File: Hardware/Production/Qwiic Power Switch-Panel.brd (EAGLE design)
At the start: 149.1 x 149.1 mm, 1505 parts, among them J1 Qwiic Right Angle, J10 PTH, J100 PTH, J103 Qwiic Right Angle, J104 PTH, J105 Qwiic Right Angle, J106 PTH, J109 Qwiic Right Angle, J110 PTH, J111 Qwiic Right Angle, J112 PTH, J115 Qwiic Right Angle, J116 PTH, J117 Qwiic Right Angle, J118 PTH, J121 Qwiic Right Angle, J122 PTH, J123 Qwiic Right Angle, J124 PTH, J127 Qwiic Right Angle, J128 PTH, J129 Qwiic Right Angle, J13 Qwiic Right Angle, J130 PTH, J133 Qwiic Right Angle, J134 PTH, J135 Qwiic Right Angle, J136 PTH, J139 Qwiic Right Angle, J14 PTH, J140 PTH, J141 Qwiic Right Angle, J142 PTH, J145 Qwiic Right Angle, J146 PTH, J147 Qwiic Right Angle, J148 PTH, J15 Qwiic Right Angle, J16 PTH, J19 Qwiic Right Angle, J2 PTH, J20 PTH, J21 Qwiic Right Angle, J22 PTH, J25 Qwiic Right Angle, J26 PTH, J27 Qwiic Right Angle, J28 PTH, J3 Qwiic Right Angle, J31 Qwiic Right Angle, J32 PTH, J33 Qwiic Right Angle, J34 PTH, J37 Qwiic Right Angle, J38 PTH, J39 Qwiic Right Angle, J4 PTH, J40 PTH, J43 Qwiic Right Angle, J44 PTH, J45 Qwiic Right Angle, J46 PTH, J49 Qwiic Right Angle, J50 PTH, J51 Qwiic Right Angle, J52 PTH, J55 Qwiic Right Angle, J56 PTH, J57 Qwiic Right Angle, J58 PTH, J61 Qwiic Right Angle, J62 PTH, J63 Qwiic Right Angle, J64 PTH, J67 Qwiic Right Angle, J68 PTH, J69 Qwiic Right Angle, J7 Qwiic Right Angle, J70 PTH, J73 Qwiic Right Angle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

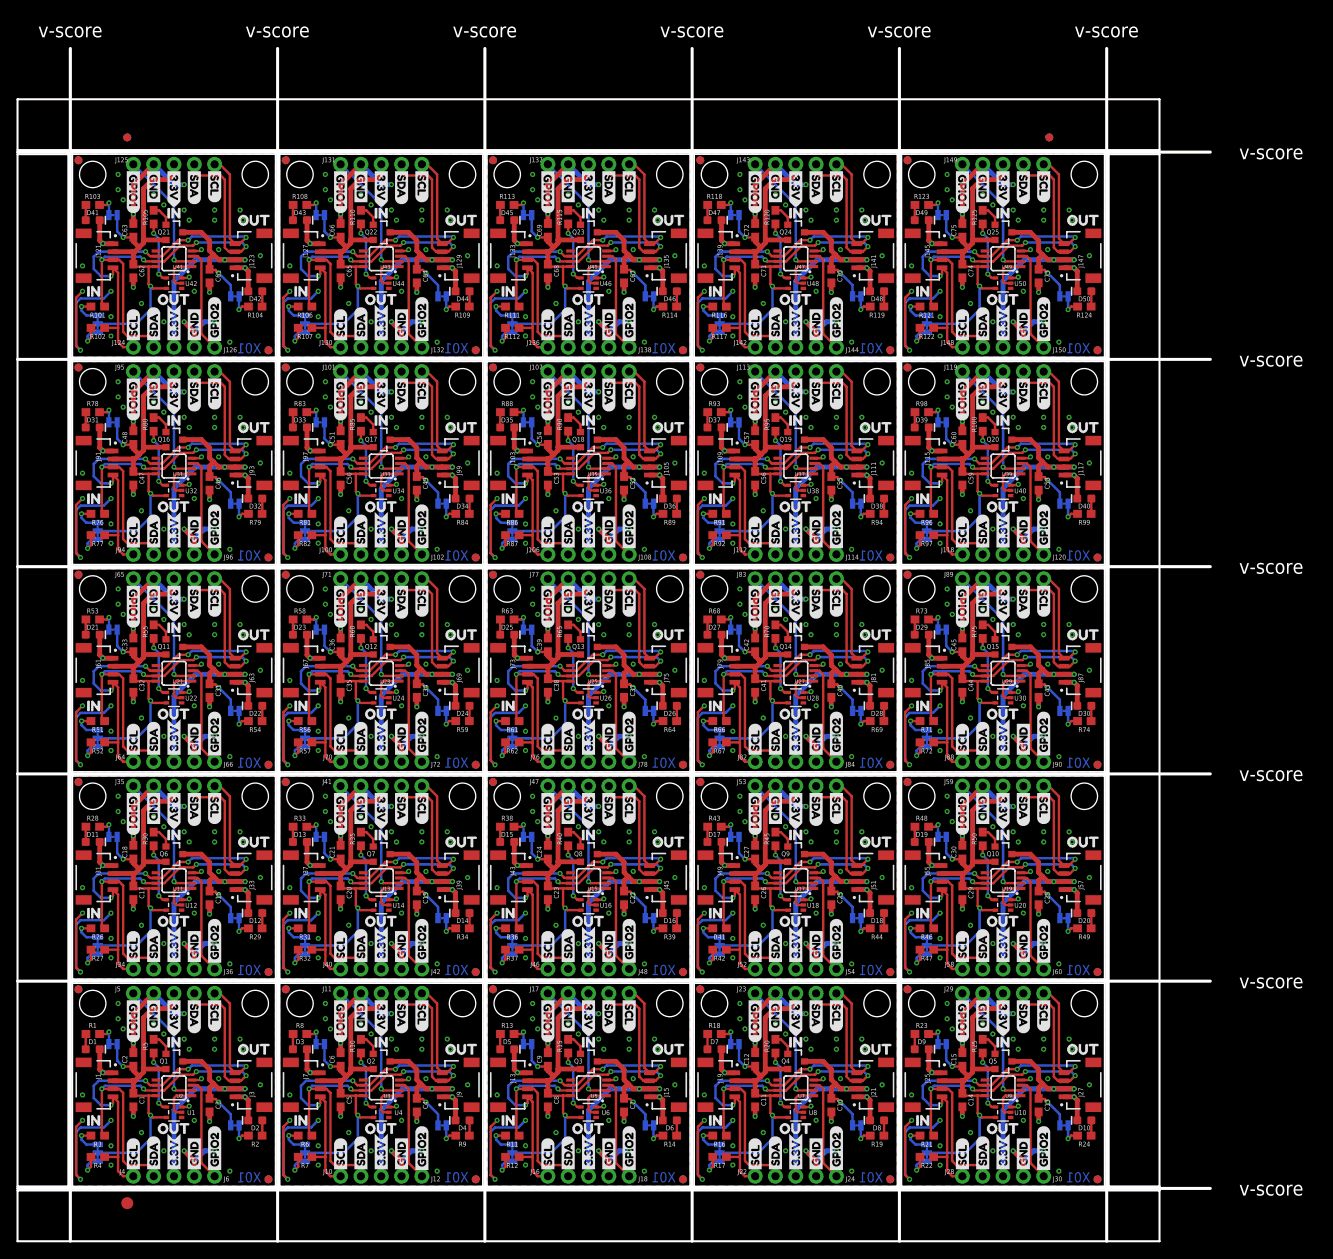
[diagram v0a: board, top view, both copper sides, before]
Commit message: Add x02 production files
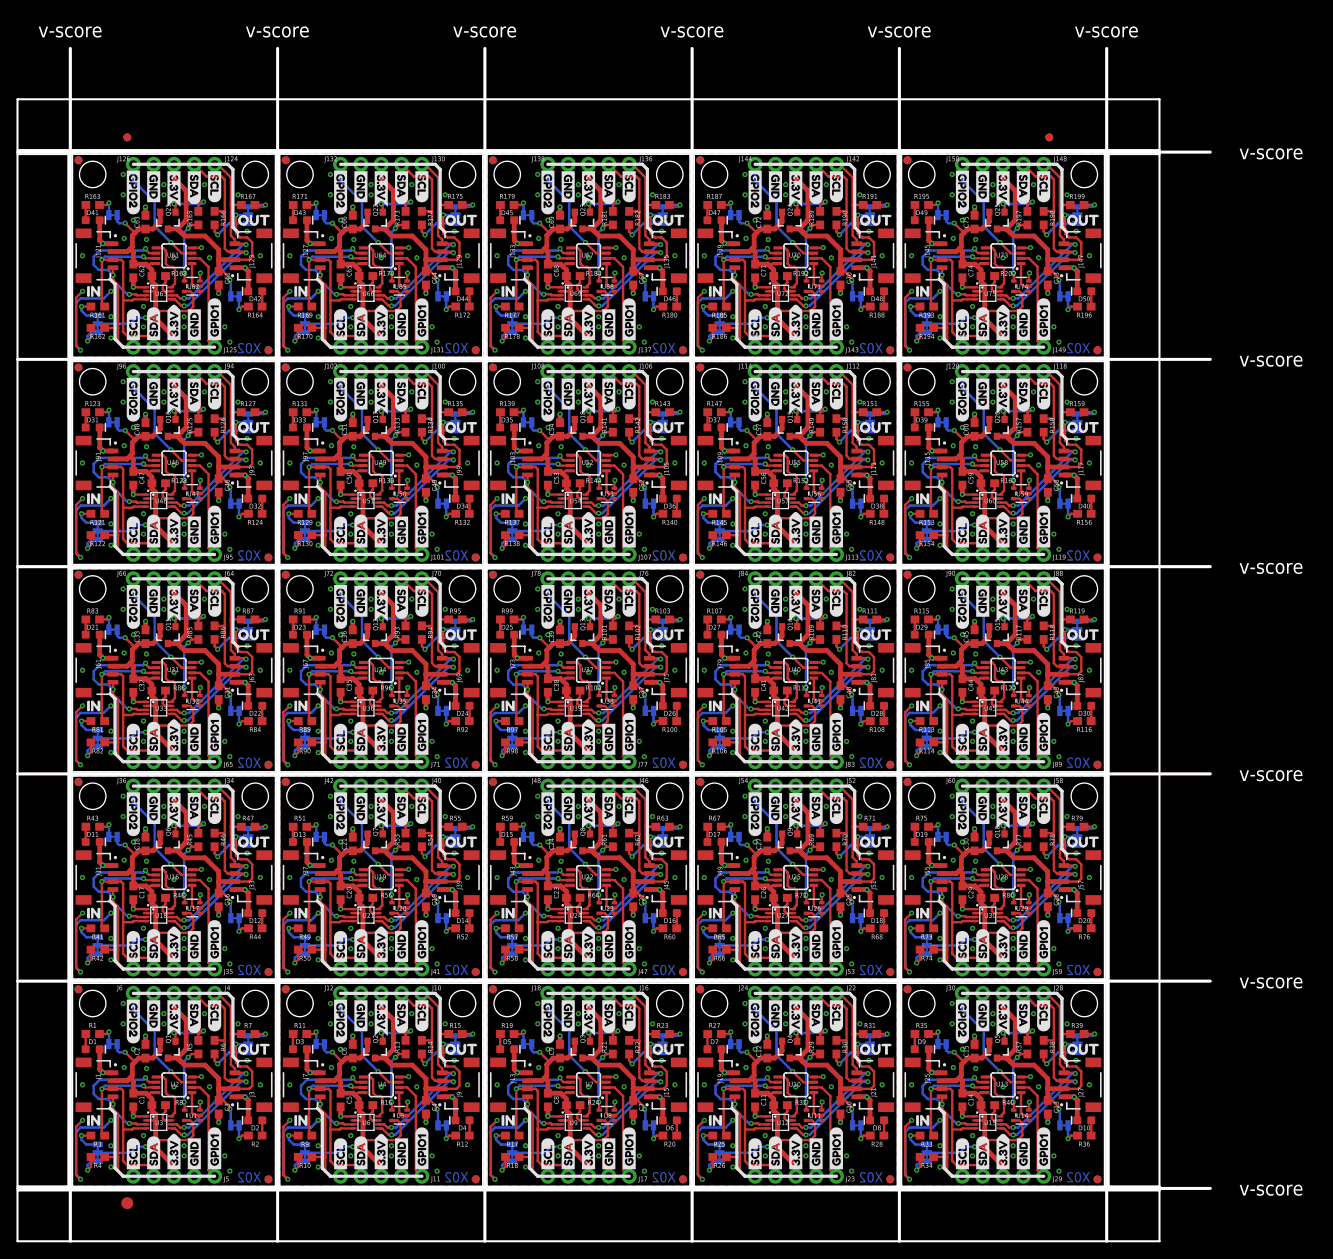
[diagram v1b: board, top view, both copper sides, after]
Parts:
- added I2C_OUT, I2C_OUT1, I2C_OUT10, I2C_OUT11, I2C_OUT12, I2C_OUT13, I2C_OUT14, I2C_OUT15, I2C_OUT16, I2C_OUT17, I2C_OUT18, I2C_OUT19, I2C_OUT2, I2C_OUT20, I2C_OUT21, I2C_OUT22, I2C_OUT23, I2C_OUT24, I2C_OUT3, I2C_OUT4, I2C_OUT5, I2C_OUT6, I2C_OUT7, I2C_OUT8, I2C_OUT9: JUMPER-SMT_3_2-NC_TRACE_SILK, SparkFun-Jumpers:SMT-JUMPER_3_2-NC_TRACE_SILK
- added R126, R127, R129, R130, R134, R135, R137, R138, R142, R143, R145, R146, R150, R151, R153, R154, R158, R159, R161, R162, R166, R167, R169, R170, R174, R175, R177, R178, R182, R183, R185, R186, R190, R191, R193, R194, R198, R199: 2.2k, SparkFun-Resistors:0603
- added R128, R136, R144, R152, R160, R168, R176, R184, R192, R200: 200k, SparkFun-Resistors:0603
- added R131, R133, R139, R141, R147, R149, R155, R157, R163, R165, R171, R173, R179, R181, R187, R189, R195, R197: 1k, SparkFun-Resistors:0603
- added R132, R140, R148, R156, R164, R172, R180, R188, R196: 470, SparkFun-Resistors:0603
- added U$776, U$800: (no value), Labels:I_SUPER2_C-()-03
- added U$777, U$780: (no value), Labels-0_04:GND1
- added U$778, U$782: (no value), Labels-0_04:SCL9
- added U$779, U$781: (no value), Labels-0_04:SDA8
- added U$783: (no value), Qwiic:QWIIC0
- added U$784, U$797: (no value), 3.3V_Flagtail:3#3V0
- added U$785, U$796: (no value), 3.3V_Pointer:3#3V0
- added U$786, U$794: (no value), GPIO1:GPIO10
- added U$787, U$795: (no value), GPIO2:GPIO20
- added U$788: (no value), IN:IN0
- added U$789: (no value), LED_IN:LED_IN0
- added U$790: (no value), LED_OUT:LED_OUT0
- added U$791: (no value), OUT:OUT0
- added U$792: (no value), Power:POWER0
- added U$793: (no value), Switch:SWITCH0
- added U$798: (no value), IN__3:IN0
- added U$799: (no value), OUT__3:OUT0
- added U51, U54, U57, U60, U63, U66, U69, U72, U75: (no value), SparkFun-IC-Comms:VSSOP_8PIN
- added U52, U55, U58, U61, U64, U67, U70, U73: PCA9536, New_Parts:MSOP8
- added U53, U56, U59, U62, U65, U68, U71, U74: 74HC1G04, SparkFun-IC-Logic:SOT353
- R10, R103, R105, R110, R113, R114, R118, R119, R14, R15, R18, R23, R25, R30, R33, R34, R38, R39, R49, R50, R54, R55, R58, R63, R65, R70, R73, R74, R78, R79, R89, R9, R90, R94, R95, R98: value 1k -> 2.2k
- R100, R108, R124, R2, R20, R28, R44, R60, R68, R84: value 1k -> 470
- R101, R107, R11, R117, R21, R27, R37, R51, R61, R67, R77, R91: value 2.2k -> 1k
- R104, R120, R24, R40, R48, R64, R8, R80, R88: value 1k -> 200k
- R112, R16, R32, R56, R72, R96: value 2.2k -> 200k
- R116, R12, R36, R52, R76, R92: value 2.2k -> 470
- U$1, U$94: value SPARKX-LOGO4 -> (none); device SparkX:SPARKX-MEDIUM -> IN__3:IN0
- U$100, U$107, U$134, U$196, U$262, U$324, U$38, U$45, U$685, U$747: device Labels-0_04:SCL9 -> Labels-0_04:SDA8
- U$101, U$194: device Labels:I_SUPER2_C-()-03 -> Labels-0_04:GND1
- U$102, U$164, U$198, U$260, U$36, U$43, U$653, U$715, U$749: device Labels-0_04:GND1 -> Labels-0_04:SDA8
- U$104, U$128, U$168, U$192, U$352, U$416: device Labels-0_04:SDA8 -> Labels:I_SUPER2_C-()-03
- U$106, U$135, U$199, U$259, U$323, U$35, U$42, U$686, U$750, U$99: device Labels-0_04:SDA8 -> Labels-0_04:SCL9
- U$108, U$201, U$325, U$418: device Qwiic:QWIIC0 -> Labels-0_04:GND1
- U$109, U$171, U$326, U$388, U$525, U$587, U$742: device 3.3V_Flagtail:3#3V0 -> Labels-0_04:SDA8
- U$110, U$234, U$327, U$451, U$462, U$586, U$679: device 3.3V_Pointer:3#3V0 -> Labels-0_04:SCL9
- U$111, U$367: device GPIO1:GPIO10 -> Qwiic:QWIIC0
- U$112, U$368, U$701: device GPIO2:GPIO20 -> 3.3V_Flagtail:3#3V0
- U$113, U$433, U$764, U$92: device IN:IN0 -> 3.3V_Pointer:3#3V0
- U$114: device LED_IN:LED_IN0 -> GPIO1:GPIO10
- U$115: device LED_OUT:LED_OUT0 -> GPIO2:GPIO20
- U$116, U$372: device OUT:OUT0 -> IN:IN0
- U$117: device Power:POWER0 -> LED_IN:LED_IN0
- U$118: device Switch:SWITCH0 -> LED_OUT:LED_OUT0
- U$119: device GPIO1:GPIO10 -> OUT:OUT0
- U$120: device GPIO2:GPIO20 -> Power:POWER0
- U$121, U$761: device 3.3V_Pointer:3#3V0 -> Switch:SWITCH0
- U$122, U$370, U$698: device 3.3V_Flagtail:3#3V0 -> GPIO1:GPIO10
- U$123, U$371, U$51: device IN:IN0 -> GPIO2:GPIO20
- U$124, U$209, U$465: device OUT:OUT0 -> 3.3V_Pointer:3#3V0
- U$125, U$528: value SPARKX-LOGO4 -> (none); device SparkX:SPARKX-MEDIUM -> 3.3V_Flagtail:3#3V0
- U$126, U$222, U$350, U$446: device Labels-0_04:GND1 -> IN__3:IN0
- U$127, U$255, U$351, U$479: device Labels-0_04:SCL9 -> OUT__3:OUT0
- U$129, U$257, U$353: value (none) -> SPARKX-LOGO4; device Labels-0_04:GND1 -> SparkX:SPARKX-MEDIUM
- U$130, U$137, U$197, U$261, U$290, U$354, U$37, U$44, U$66, U$73, U$748: device Labels-0_04:SDA8 -> Labels-0_04:GND1
- U$132, U$70: device Labels:I_SUPER2_C-()-03 -> Labels-0_04:SDA8
- U$136, U$160, U$18, U$288, U$384, U$40, U$64: device Labels-0_04:GND1 -> Labels:I_SUPER2_C-()-03
- U$139, U$294, U$356, U$77: device Qwiic:QWIIC0 -> Labels-0_04:SDA8
- U$14, U$671: device IN:IN0 -> OUT__3:OUT0
- U$140, U$233, U$357, U$450, U$556, U$649, U$773: device 3.3V_Flagtail:3#3V0 -> Labels-0_04:GND1
- U$141, U$203, U$358, U$420, U$493, U$555, U$710, U$772: device 3.3V_Pointer:3#3V0 -> Labels-0_04:SDA8
- U$142, U$266, U$359, U$398, U$483, U$522, U$615, U$739: device GPIO1:GPIO10 -> Labels-0_04:SCL9
- U$143, U$399: device GPIO2:GPIO20 -> Qwiic:QWIIC0
- U$144, U$464, U$61, U$733: device IN:IN0 -> 3.3V_Flagtail:3#3V0
- U$145: device LED_IN:LED_IN0 -> 3.3V_Pointer:3#3V0
- U$146: device LED_OUT:LED_OUT0 -> GPIO1:GPIO10
- U$147, U$155, U$403: device OUT:OUT0 -> GPIO2:GPIO20
- U$148: device Power:POWER0 -> IN:IN0
- U$149: device Switch:SWITCH0 -> LED_IN:LED_IN0
- U$150: device GPIO1:GPIO10 -> LED_OUT:LED_OUT0
- U$151: device GPIO2:GPIO20 -> OUT:OUT0
- U$152: device 3.3V_Pointer:3#3V0 -> Power:POWER0
- U$153, U$729: device 3.3V_Flagtail:3#3V0 -> Switch:SWITCH0
- U$154, U$402, U$82: device IN:IN0 -> GPIO1:GPIO10
- U$156, U$497: value SPARKX-LOGO4 -> (none); device SparkX:SPARKX-MEDIUM -> 3.3V_Pointer:3#3V0
- U$157, U$253, U$381, U$477, U$560, U$656: device Labels-0_04:GND1 -> 3.3V_Flagtail:3#3V0
- U$158, U$286, U$382, U$510: device Labels-0_04:SCL9 -> IN__3:IN0
- U$159, U$223, U$383, U$447: device Labels-0_04:SDA8 -> OUT__3:OUT0
- U$161, U$321, U$385, U$97: value (none) -> SPARKX-LOGO4; device Labels-0_04:SDA8 -> SparkX:SPARKX-MEDIUM
- U$162, U$165, U$169, U$258, U$293, U$33, U$386, U$41, U$69, U$716, U$76: device Labels-0_04:SCL9 -> Labels-0_04:GND1
- U$163, U$39: device Labels:I_SUPER2_C-()-03 -> Labels-0_04:SCL9
- U$167, U$195, U$291, U$622, U$67, U$71, U$718, U$74, U$746: device Labels-0_04:GND1 -> Labels-0_04:SCL9
- U$170, U$263, U$387, U$46: device Qwiic:QWIIC0 -> Labels-0_04:SCL9
- U$172, U$265, U$389, U$482, U$524, U$617, U$741: device 3.3V_Pointer:3#3V0 -> Labels-0_04:GND1
- U$173, U$235, U$390, U$429, U$452, U$491, U$646, U$708: device GPIO1:GPIO10 -> Labels-0_04:SDA8
- U$174, U$298, U$391, U$430, U$515, U$554, U$647, U$771: device GPIO2:GPIO20 -> Labels-0_04:SCL9
- U$175, U$495: device IN:IN0 -> Qwiic:QWIIC0
- U$176, U$765: device LED_IN:LED_IN0 -> 3.3V_Flagtail:3#3V0
- U$177: device LED_OUT:LED_OUT0 -> 3.3V_Pointer:3#3V0
- U$178, U$186, U$434: device OUT:OUT0 -> GPIO1:GPIO10
- U$179: device Power:POWER0 -> GPIO2:GPIO20
- U$180: device Switch:SWITCH0 -> IN:IN0
- U$181: device GPIO1:GPIO10 -> LED_IN:LED_IN0
- U$182: device GPIO2:GPIO20 -> LED_OUT:LED_OUT0
- U$183: device 3.3V_Pointer:3#3V0 -> OUT:OUT0
- U$184, U$760: device 3.3V_Flagtail:3#3V0 -> Power:POWER0
- U$185: device IN:IN0 -> Switch:SWITCH0
- U$187, U$435: value SPARKX-LOGO4 -> (none); device SparkX:SPARKX-MEDIUM -> GPIO2:GPIO20
- U$188, U$284, U$412, U$508, U$529, U$625, U$753: device Labels-0_04:GND1 -> 3.3V_Pointer:3#3V0
- U$189, U$317, U$413, U$541, U$592, U$720: device Labels-0_04:SCL9 -> 3.3V_Flagtail:3#3V0
- U$190, U$254, U$414, U$478: device Labels-0_04:SDA8 -> IN__3:IN0
- U$191, U$319, U$415, U$95: device Labels-0_04:GND1 -> OUT__3:OUT0
- U$193, U$289, U$417, U$65: value (none) -> SPARKX-LOGO4; device Labels-0_04:SCL9 -> SparkX:SPARKX-MEDIUM
- U$200, U$224, U$320, U$448, U$72, U$96: device Labels-0_04:SCL9 -> Labels:I_SUPER2_C-()-03
- U$202, U$295, U$419, U$494, U$618, U$711, U$78: device 3.3V_Flagtail:3#3V0 -> Labels-0_04:SCL9
- U$204, U$297, U$421, U$460, U$514, U$553, U$677, U$770: device GPIO1:GPIO10 -> Labels-0_04:GND1
- U$205, U$267, U$422, U$461, U$484, U$523, U$678, U$740: device GPIO2:GPIO20 -> Labels-0_04:SDA8
- U$206, U$330, U$423, U$526, U$547, U$650, U$743: device IN:IN0 -> Labels-0_04:SCL9
- U$207: device LED_IN:LED_IN0 -> Qwiic:QWIIC0
- U$208: device LED_OUT:LED_OUT0 -> 3.3V_Flagtail:3#3V0
- U$21, U$705: value (none) -> SPARKX-LOGO4; device OUT:OUT0 -> SparkX:SPARKX-MEDIUM
- U$210: device Power:POWER0 -> GPIO1:GPIO10
- U$211: device Switch:SWITCH0 -> GPIO2:GPIO20
- U$212: device GPIO1:GPIO10 -> IN:IN0
- U$213: device GPIO2:GPIO20 -> LED_IN:LED_IN0
- U$214: device 3.3V_Pointer:3#3V0 -> LED_OUT:LED_OUT0
- U$215: device 3.3V_Flagtail:3#3V0 -> OUT:OUT0
- U$216: device IN:IN0 -> Power:POWER0
- U$217: device OUT:OUT0 -> Switch:SWITCH0
- U$218, U$466: value SPARKX-LOGO4 -> (none); device SparkX:SPARKX-MEDIUM -> GPIO1:GPIO10
- U$219, U$315, U$443, U$467, U$539, U$563, U$691: device Labels-0_04:GND1 -> GPIO2:GPIO20
- U$220, U$348, U$444, U$561, U$572, U$689: device Labels-0_04:SCL9 -> 3.3V_Pointer:3#3V0
- U$221, U$285, U$445, U$509, U$624, U$688: device Labels-0_04:SDA8 -> 3.3V_Flagtail:3#3V0
- U$225: value (none) -> SPARKX-LOGO4; device Labels:I_SUPER2_C-()-03 -> SparkX:SPARKX-MEDIUM
- U$232, U$480: device Qwiic:QWIIC0 -> Labels:I_SUPER2_C-()-03
- U$236, U$329, U$453, U$492, U$546, U$585, U$709: device GPIO2:GPIO20 -> Labels-0_04:GND1
- U$237, U$299, U$454, U$516, U$557, U$619, U$774: device IN:IN0 -> Labels-0_04:SDA8
- U$238, U$362, U$455, U$579: device LED_IN:LED_IN0 -> Labels-0_04:SCL9
- U$239: device LED_OUT:LED_OUT0 -> Qwiic:QWIIC0
- U$240, U$496, U$93: device OUT:OUT0 -> 3.3V_Flagtail:3#3V0
- U$241: device Power:POWER0 -> 3.3V_Pointer:3#3V0
- U$242: device Switch:SWITCH0 -> GPIO1:GPIO10
- U$243, U$731: device GPIO1:GPIO10 -> GPIO2:GPIO20
- U$244: device GPIO2:GPIO20 -> IN:IN0
- U$245: device 3.3V_Pointer:3#3V0 -> LED_IN:LED_IN0
- U$246: device 3.3V_Flagtail:3#3V0 -> LED_OUT:LED_OUT0
- U$247: device IN:IN0 -> OUT:OUT0
- U$248: device OUT:OUT0 -> Power:POWER0
- U$249: value SPARKX-LOGO4 -> (none); device SparkX:SPARKX-MEDIUM -> Switch:SWITCH0
- U$250, U$346, U$474, U$498, U$570, U$594, U$722: device Labels-0_04:GND1 -> GPIO1:GPIO10
- U$251, U$379, U$475, U$499, U$603, U$627, U$723: device Labels-0_04:SCL9 -> GPIO2:GPIO20
- U$252, U$316, U$476, U$540, U$593, U$657: device Labels-0_04:SDA8 -> 3.3V_Pointer:3#3V0
- U$264, U$512, U$680: device 3.3V_Flagtail:3#3V0 -> Labels:I_SUPER2_C-()-03
- U$268, U$361, U$485, U$578, U$588, U$681: device IN:IN0 -> Labels-0_04:GND1
- U$269, U$331, U$486, U$548: device LED_IN:LED_IN0 -> Labels-0_04:SDA8
- U$270, U$394, U$487, U$611: device LED_OUT:LED_OUT0 -> Labels-0_04:SCL9
- U$271, U$527: device OUT:OUT0 -> Qwiic:QWIIC0
- U$272: device Power:POWER0 -> 3.3V_Flagtail:3#3V0
- U$273: device Switch:SWITCH0 -> 3.3V_Pointer:3#3V0
- U$276: device 3.3V_Pointer:3#3V0 -> IN:IN0
- U$277: device 3.3V_Flagtail:3#3V0 -> LED_IN:LED_IN0
- U$278: device IN:IN0 -> LED_OUT:LED_OUT0
- U$280: value SPARKX-LOGO4 -> (none); device SparkX:SPARKX-MEDIUM -> Power:POWER0
- U$281, U$377, U$505, U$601: device Labels-0_04:GND1 -> Switch:SWITCH0
- U$282, U$410, U$506, U$530, U$634, U$658, U$754: device Labels-0_04:SCL9 -> GPIO1:GPIO10
- U$283, U$347, U$507, U$531, U$571, U$595, U$755: device Labels-0_04:SDA8 -> GPIO2:GPIO20
- U$287: device Labels:I_SUPER2_C-()-03 -> OUT__3:OUT0
- U$296, U$544, U$648: device 3.3V_Pointer:3#3V0 -> Labels:I_SUPER2_C-()-03
- U$300, U$393, U$517, U$610: device LED_IN:LED_IN0 -> Labels-0_04:GND1
- U$301, U$363, U$518, U$580: device LED_OUT:LED_OUT0 -> Labels-0_04:SDA8
- U$302, U$426, U$519, U$558, U$643, U$682, U$775: device OUT:OUT0 -> Labels-0_04:SCL9
- U$303: device Power:POWER0 -> Qwiic:QWIIC0
- U$304: device Switch:SWITCH0 -> 3.3V_Flagtail:3#3V0
- U$305, U$49, U$700: device GPIO1:GPIO10 -> 3.3V_Pointer:3#3V0
- U$306, U$50, U$58: device GPIO2:GPIO20 -> GPIO1:GPIO10
- U$307, U$59, U$699: device 3.3V_Pointer:3#3V0 -> GPIO2:GPIO20
- U$308: device 3.3V_Flagtail:3#3V0 -> IN:IN0
- U$309: device IN:IN0 -> LED_IN:LED_IN0
- U$310, U$54: device OUT:OUT0 -> LED_OUT:LED_OUT0
- U$311: value SPARKX-LOGO4 -> (none); device SparkX:SPARKX-MEDIUM -> OUT:OUT0
- U$312, U$408, U$536, U$632: device Labels-0_04:GND1 -> Power:POWER0
- U$313, U$441, U$537, U$665: device Labels-0_04:SCL9 -> Switch:SWITCH0
- U$314, U$378, U$538, U$562, U$602, U$626: device Labels-0_04:SDA8 -> GPIO1:GPIO10
- U$318: device Labels:I_SUPER2_C-()-03 -> IN__3:IN0
- U$328, U$576, U$584: device GPIO1:GPIO10 -> Labels:I_SUPER2_C-()-03
- U$332, U$425, U$549, U$642: device LED_OUT:LED_OUT0 -> Labels-0_04:GND1
- U$333, U$395, U$550, U$589, U$612, U$651: device OUT:OUT0 -> Labels-0_04:SDA8
- U$334, U$458, U$551, U$675: device Power:POWER0 -> Labels-0_04:SCL9
- U$335: device Switch:SWITCH0 -> Qwiic:QWIIC0
- U$336, U$669, U$80: device GPIO1:GPIO10 -> 3.3V_Flagtail:3#3V0
- U$337, U$732, U$81: device GPIO2:GPIO20 -> 3.3V_Pointer:3#3V0
- U$338, U$730, U$90: device 3.3V_Pointer:3#3V0 -> GPIO1:GPIO10
- U$339, U$667, U$91: device 3.3V_Flagtail:3#3V0 -> GPIO2:GPIO20
- U$341, U$85: device OUT:OUT0 -> LED_IN:LED_IN0
- U$342: value SPARKX-LOGO4 -> (none); device SparkX:SPARKX-MEDIUM -> LED_OUT:LED_OUT0
- U$343, U$439, U$567, U$663: device Labels-0_04:GND1 -> OUT:OUT0
- U$344, U$472, U$568, U$696: device Labels-0_04:SCL9 -> Power:POWER0
- U$345, U$409, U$569, U$633: device Labels-0_04:SDA8 -> Switch:SWITCH0
- U$349, U$752: device Labels:I_SUPER2_C-()-03 -> 3.3V_Flagtail:3#3V0
- U$360, U$608, U$616: device GPIO2:GPIO20 -> Labels:I_SUPER2_C-()-03
- U$364, U$457, U$581, U$620, U$674, U$713: device OUT:OUT0 -> Labels-0_04:GND1
- U$365, U$427, U$582, U$644: device Power:POWER0 -> Labels-0_04:SDA8
- U$366, U$490, U$583, U$707: device Switch:SWITCH0 -> Labels-0_04:SCL9
- U$373: value SPARKX-LOGO4 -> (none); device SparkX:SPARKX-MEDIUM -> LED_IN:LED_IN0
- U$374, U$470, U$598, U$694: device Labels-0_04:GND1 -> LED_OUT:LED_OUT0
- U$375, U$503, U$599, U$727: device Labels-0_04:SCL9 -> OUT:OUT0
- U$376, U$440, U$600, U$664: device Labels-0_04:SDA8 -> Power:POWER0
- U$380, U$721: device Labels:I_SUPER2_C-()-03 -> 3.3V_Pointer:3#3V0
- U$392, U$640, U$712: device IN:IN0 -> Labels:I_SUPER2_C-()-03
- U$396, U$489, U$613, U$706: device Power:POWER0 -> Labels-0_04:GND1
- U$397, U$459, U$614, U$676: device Switch:SWITCH0 -> Labels-0_04:SDA8
- U$400, U$48, U$637: device 3.3V_Pointer:3#3V0 -> 3.3V_Flagtail:3#3V0
- U$401, U$60, U$636: device 3.3V_Flagtail:3#3V0 -> 3.3V_Pointer:3#3V0
- U$404: value SPARKX-LOGO4 -> (none); device SparkX:SPARKX-MEDIUM -> IN:IN0
- U$405, U$501, U$629, U$725: device Labels-0_04:GND1 -> LED_IN:LED_IN0
- U$406, U$534, U$630, U$758: device Labels-0_04:SCL9 -> LED_OUT:LED_OUT0
- U$407, U$471, U$631, U$695: device Labels-0_04:SDA8 -> OUT:OUT0
- U$411, U$659: device Labels:I_SUPER2_C-()-03 -> GPIO2:GPIO20
- U$424, U$672: device LED_IN:LED_IN0 -> Labels:I_SUPER2_C-()-03
- U$428, U$521, U$645, U$738: device Switch:SWITCH0 -> Labels-0_04:GND1
- U$431, U$79: device 3.3V_Pointer:3#3V0 -> Qwiic:QWIIC0
- U$436, U$532, U$660, U$756: device Labels-0_04:GND1 -> IN:IN0
- U$437, U$565, U$661: device Labels-0_04:SCL9 -> LED_IN:LED_IN0
- U$438, U$502, U$662, U$726: device Labels-0_04:SDA8 -> LED_OUT:LED_OUT0
- U$442, U$690: device Labels:I_SUPER2_C-()-03 -> GPIO1:GPIO10
- U$449: value (none) -> SPARKX-LOGO4; device Qwiic:QWIIC0 -> SparkX:SPARKX-MEDIUM
- U$456, U$704: device LED_OUT:LED_OUT0 -> Labels:I_SUPER2_C-()-03
- U$463, U$47: device 3.3V_Flagtail:3#3V0 -> Qwiic:QWIIC0
- U$468, U$596, U$692: device Labels-0_04:SCL9 -> IN:IN0
- U$469, U$533, U$693, U$757: device Labels-0_04:SDA8 -> LED_IN:LED_IN0
- U$473: device Labels:I_SUPER2_C-()-03 -> Switch:SWITCH0
- U$481: value (none) -> SPARKX-LOGO4; device 3.3V_Flagtail:3#3V0 -> SparkX:SPARKX-MEDIUM
- U$488, U$736, U$744: device OUT:OUT0 -> Labels:I_SUPER2_C-()-03
- U$500, U$564, U$724: device Labels-0_04:SDA8 -> IN:IN0
- U$504: device Labels:I_SUPER2_C-()-03 -> Power:POWER0
- U$511: device Qwiic:QWIIC0 -> OUT__3:OUT0
- U$513: value (none) -> SPARKX-LOGO4; device 3.3V_Pointer:3#3V0 -> SparkX:SPARKX-MEDIUM
- U$52: device LED_IN:LED_IN0 -> IN:IN0
- U$520, U$768: device Power:POWER0 -> Labels:I_SUPER2_C-()-03
- U$53: device LED_OUT:LED_OUT0 -> LED_IN:LED_IN0
- U$535: device Labels:I_SUPER2_C-()-03 -> OUT:OUT0
- U$542: device Qwiic:QWIIC0 -> IN__3:IN0
- U$543: device 3.3V_Flagtail:3#3V0 -> OUT__3:OUT0
- U$545: value (none) -> SPARKX-LOGO4; device GPIO1:GPIO10 -> SparkX:SPARKX-MEDIUM
- U$55: device Power:POWER0 -> OUT:OUT0
- U$552: device Switch:SWITCH0 -> Labels:I_SUPER2_C-()-03
- U$559: value SPARKX-LOGO4 -> (none); device SparkX:SPARKX-MEDIUM -> Qwiic:QWIIC0
- U$56: device Switch:SWITCH0 -> Power:POWER0
- U$566: device Labels:I_SUPER2_C-()-03 -> LED_OUT:LED_OUT0
- U$57: device GPIO1:GPIO10 -> Switch:SWITCH0
- U$573: device Qwiic:QWIIC0 -> 3.3V_Flagtail:3#3V0
- U$574: device 3.3V_Flagtail:3#3V0 -> IN__3:IN0
- U$575: device 3.3V_Pointer:3#3V0 -> OUT__3:OUT0
- U$577: value (none) -> SPARKX-LOGO4; device GPIO2:GPIO20 -> SparkX:SPARKX-MEDIUM
- U$590, U$714: value SPARKX-LOGO4 -> (none); device SparkX:SPARKX-MEDIUM -> Labels-0_04:SCL9
- U$591, U$687: device Labels-0_04:GND1 -> Qwiic:QWIIC0
- U$597: device Labels:I_SUPER2_C-()-03 -> LED_IN:LED_IN0
- U$604: device Qwiic:QWIIC0 -> 3.3V_Pointer:3#3V0
- U$606: device 3.3V_Pointer:3#3V0 -> IN__3:IN0
- U$607: device GPIO1:GPIO10 -> OUT__3:OUT0
- U$609: value (none) -> SPARKX-LOGO4; device IN:IN0 -> SparkX:SPARKX-MEDIUM
- U$62: device OUT:OUT0 -> IN__3:IN0
- U$621, U$683: value SPARKX-LOGO4 -> (none); device SparkX:SPARKX-MEDIUM -> Labels-0_04:SDA8
- U$623, U$751: device Labels-0_04:SCL9 -> Qwiic:QWIIC0
- U$628: device Labels:I_SUPER2_C-()-03 -> IN:IN0
- U$63: value SPARKX-LOGO4 -> (none); device SparkX:SPARKX-MEDIUM -> OUT__3:OUT0
- U$635: device Qwiic:QWIIC0 -> GPIO2:GPIO20
- U$638: device GPIO1:GPIO10 -> IN__3:IN0
- U$639: device GPIO2:GPIO20 -> OUT__3:OUT0
- U$641: value (none) -> SPARKX-LOGO4; device LED_IN:LED_IN0 -> SparkX:SPARKX-MEDIUM
- U$652, U$745: value SPARKX-LOGO4 -> (none); device SparkX:SPARKX-MEDIUM -> Labels-0_04:GND1
- U$655, U$719: device Labels-0_04:SDA8 -> Qwiic:QWIIC0
- U$666: device Qwiic:QWIIC0 -> GPIO1:GPIO10
- U$670: device GPIO2:GPIO20 -> IN__3:IN0
- U$673: value (none) -> SPARKX-LOGO4; device LED_OUT:LED_OUT0 -> SparkX:SPARKX-MEDIUM
- U$697: device Qwiic:QWIIC0 -> Switch:SWITCH0
- U$702: device IN:IN0 -> IN__3:IN0
- U$703: device LED_IN:LED_IN0 -> OUT__3:OUT0
- U$728: device Qwiic:QWIIC0 -> Power:POWER0
- U$734: device LED_IN:LED_IN0 -> IN__3:IN0
- U$735: device LED_OUT:LED_OUT0 -> OUT__3:OUT0
- U$737: value (none) -> SPARKX-LOGO4; device Power:POWER0 -> SparkX:SPARKX-MEDIUM
- U$759: device Qwiic:QWIIC0 -> OUT:OUT0
- U$766: device LED_OUT:LED_OUT0 -> IN__3:IN0
- U$767: device OUT:OUT0 -> OUT__3:OUT0
- U$769: value (none) -> SPARKX-LOGO4; device Switch:SWITCH0 -> SparkX:SPARKX-MEDIUM
- U$83: device LED_IN:LED_IN0 -> GPIO2:GPIO20
- U$84: device LED_OUT:LED_OUT0 -> IN:IN0
- U$86: device Power:POWER0 -> LED_OUT:LED_OUT0
- U$87: device Switch:SWITCH0 -> OUT:OUT0
- U$88: device GPIO1:GPIO10 -> Power:POWER0
- U$89: device GPIO2:GPIO20 -> Switch:SWITCH0
- U10, U16, U22, U28, U34, U4, U40, U46: value 74HC1G04 -> PCA9536; device SparkFun-IC-Logic:SOT353 -> New_Parts:MSOP8
- U11, U17, U23, U29, U35, U41, U47, U5: value PCA9536 -> 74HC1G04; device New_Parts:MSOP8 -> SparkFun-IC-Logic:SOT353
- U12, U18, U24, U30, U36, U42, U48, U6: value 74HC1G04 -> (none); device SparkFun-IC-Logic:SOT353 -> SparkFun-IC-Comms:VSSOP_8PIN
- U15, U21, U27, U3, U33, U39, U45, U9: value PCA9536 -> (none); device New_Parts:MSOP8 -> SparkFun-IC-Comms:VSSOP_8PIN
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- renumbered I2C to I2C_IN, I2C1 to I2C_IN1, I2C10 to I2C_IN10, I2C11 to I2C_IN11, I2C12 to I2C_IN12, I2C13 to I2C_IN13, I2C14 to I2C_IN14, I2C15 to I2C_IN15, I2C16 to I2C_IN16, I2C17 to I2C_IN17, I2C18 to I2C_IN18, I2C19 to I2C_IN19, I2C2 to I2C_IN2, I2C20 to I2C_IN20, I2C21 to I2C_IN21, I2C22 to I2C_IN22, I2C23 to I2C_IN23, I2C24 to I2C_IN24, I2C3 to I2C_IN3, I2C4 to I2C_IN4, I2C5 to I2C_IN5, I2C6 to I2C_IN6, I2C7 to I2C_IN7, I2C8 to I2C_IN8, I2C9 to I2C_IN9
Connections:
- new net GPIO75: U55.5, U57.P8
- new net GPIO76: U58.1, U59.2
- new net GPIO77: J119.1, U58.2
- new net GPIO78: J120.1, U58.3
- new net GPIO79: U58.5, U60.P8
- new net GPIO80: U61.1, U62.2
- new net GPIO81: J125.1, U61.2
- new net GPIO82: J126.1, U61.3
- new net GPIO83: U61.5, U63.P8
- new net GPIO84: U64.1, U65.2
- new net GPIO85: J131.1, U64.2
- new net GPIO86: J132.1, U64.3
- new net GPIO87: U64.5, U66.P8
- new net GPIO88: U67.1, U68.2
- new net GPIO89: J137.1, U67.2
- new net GPIO90: J138.1, U67.3
- new net GPIO91: U67.5, U69.P8
- new net GPIO92: U70.1, U71.2
- new net GPIO93: J143.1, U70.2
- new net GPIO94: J144.1, U70.3
- new net GPIO95: U70.5, U72.P8
- new net GPIO96: U73.1, U74.2
- new net GPIO97: J149.1, U73.2
- new net GPIO98: J150.1, U73.3
- new net GPIO99: U73.5, U75.P8
- new net N$201: D37.A, R147.1
- new net N$202: D38.A, R148.1
- new net N$203: IN_LED18.1, R147.2
- new net N$204: OUT_LED18.1, R148.2
- new net N$205: R149.1, U56.4
- new net N$206: Q19.1, R149.2
- new net N$207: I2C_OUT18.1, R151.2
- new net N$208: I2C_OUT18.3, R150.2
- new net N$209: R152.1, U57.P7
- new net N$210: I2C_IN19.1, R154.2
- new net N$211: I2C_IN19.3, R153.2
- new net N$212: D39.A, R155.1
- new net N$213: D40.A, R156.1
- new net N$214: IN_LED19.1, R155.2
- new net N$215: OUT_LED19.1, R156.2
- new net N$216: R157.1, U59.4
- new net N$217: Q20.1, R157.2
- new net N$218: I2C_OUT19.1, R159.2
- new net N$219: I2C_OUT19.3, R158.2
- new net N$220: R160.1, U60.P7
- new net N$221: I2C_IN20.1, R162.2
- new net N$222: I2C_IN20.3, R161.2
- new net N$223: D41.A, R163.1
- new net N$224: D42.A, R164.1
- new net N$225: IN_LED20.1, R163.2
- new net N$226: OUT_LED20.1, R164.2
- new net N$227: R165.1, U62.4
- new net N$228: Q21.1, R165.2
- new net N$229: I2C_OUT20.1, R167.2
- new net N$230: I2C_OUT20.3, R166.2
- new net N$231: R168.1, U63.P7
- new net N$232: I2C_IN21.1, R170.2
- new net N$233: I2C_IN21.3, R169.2
- new net N$234: D43.A, R171.1
- new net N$235: D44.A, R172.1
- new net N$236: IN_LED21.1, R171.2
- new net N$237: OUT_LED21.1, R172.2
- new net N$238: R173.1, U65.4
- new net N$239: Q22.1, R173.2
- new net N$240: I2C_OUT21.1, R175.2
- new net N$241: I2C_OUT21.3, R174.2
- new net N$242: R176.1, U66.P7
- new net N$243: I2C_IN22.1, R178.2
- new net N$244: I2C_IN22.3, R177.2
- new net N$245: D45.A, R179.1
- new net N$246: D46.A, R180.1
- new net N$247: IN_LED22.1, R179.2
- new net N$248: OUT_LED22.1, R180.2
- new net N$249: R181.1, U68.4
- new net N$250: Q23.1, R181.2
- new net N$251: I2C_OUT22.1, R183.2
- new net N$252: I2C_OUT22.3, R182.2
- new net N$253: R184.1, U69.P7
- new net N$254: I2C_IN23.1, R186.2
- new net N$255: I2C_IN23.3, R185.2
- new net N$256: D47.A, R187.1
- new net N$257: D48.A, R188.1
- new net N$258: IN_LED23.1, R187.2
- new net N$259: OUT_LED23.1, R188.2
- new net N$260: R189.1, U71.4
- new net N$261: Q24.1, R189.2
- new net N$262: I2C_OUT23.1, R191.2
- new net N$263: I2C_OUT23.3, R190.2
- new net N$264: R192.1, U72.P7
- new net N$265: I2C_IN24.1, R194.2
- new net N$266: I2C_IN24.3, R193.2
- new net N$267: D49.A, R195.1
- new net N$268: D50.A, R196.1
- new net N$269: IN_LED24.1, R195.2
- new net N$270: OUT_LED24.1, R196.2
- new net N$271: R197.1, U74.4
- new net N$272: Q25.1, R197.2
- new net N$273: I2C_OUT24.1, R199.2
- new net N$274: I2C_OUT24.3, R198.2
- new net N$275: R200.1, U75.P7
- new net SCL_OUT: J3.4, J4.4, R7.1, U3.P6
- new net SCL_OUT1: J10.4, J9.4, R15.1, U6.P6
- new net SCL_OUT10: J63.4, J64.4, R87.1, U33.P6
- new net SCL_OUT11: J69.4, J70.4, R95.1, U36.P6
- new net SCL_OUT12: J75.4, J76.4, R103.1, U39.P6
- new net SCL_OUT13: J81.4, J82.4, R111.1, U42.P6
- new net SCL_OUT14: J87.4, J88.4, R119.1, U45.P6
- new net SCL_OUT15: J93.4, J94.4, R127.1, U48.P6
- new net SCL_OUT16: J100.4, J99.4, R135.1, U51.P6
- new net SCL_OUT17: J105.4, J106.4, R143.1, U54.P6
- new net SCL_OUT18: J111.4, J112.4, R151.1, U57.P6
- new net SCL_OUT19: J117.4, J118.4, R159.1, U60.P6
- new net SCL_OUT2: J15.4, J16.4, R23.1, U9.P6
- new net SCL_OUT20: J123.4, J124.4, R167.1, U63.P6
- new net SCL_OUT21: J129.4, J130.4, R175.1, U66.P6
- new net SCL_OUT22: J135.4, J136.4, R183.1, U69.P6
- new net SCL_OUT23: J141.4, J142.4, R191.1, U72.P6
- new net SCL_OUT24: J147.4, J148.4, R199.1, U75.P6
- new net SCL_OUT3: J21.4, J22.4, R31.1, U12.P6
- new net SCL_OUT4: J27.4, J28.4, R39.1, U15.P6
- new net SCL_OUT5: J33.4, J34.4, R47.1, U18.P6
- new net SCL_OUT6: J39.4, J40.4, R55.1, U21.P6
- new net SCL_OUT7: J45.4, J46.4, R63.1, U24.P6
- new net SCL_OUT8: J51.4, J52.4, R71.1, U27.P6
- new net SCL_OUT9: J57.4, J58.4, R79.1, U30.P6
- new net SDA_OUT: J3.3, J4.3, R6.1, U3.P5
- new net SDA_OUT1: J10.3, J9.3, R14.1, U6.P5
- new net SDA_OUT10: J63.3, J64.3, R86.1, U33.P5
- new net SDA_OUT11: J69.3, J70.3, R94.1, U36.P5
- new net SDA_OUT12: J75.3, J76.3, R102.1, U39.P5
- new net SDA_OUT13: J81.3, J82.3, R110.1, U42.P5
- new net SDA_OUT14: J87.3, J88.3, R118.1, U45.P5
- new net SDA_OUT15: J93.3, J94.3, R126.1, U48.P5
- new net SDA_OUT16: J100.3, J99.3, R134.1, U51.P5
- new net SDA_OUT17: J105.3, J106.3, R142.1, U54.P5
- new net SDA_OUT18: J111.3, J112.3, R150.1, U57.P5
- new net SDA_OUT19: J117.3, J118.3, R158.1, U60.P5
- new net SDA_OUT2: J15.3, J16.3, R22.1, U9.P5
- new net SDA_OUT20: J123.3, J124.3, R166.1, U63.P5
- new net SDA_OUT21: J129.3, J130.3, R174.1, U66.P5
- new net SDA_OUT22: J135.3, J136.3, R182.1, U69.P5
- new net SDA_OUT23: J141.3, J142.3, R190.1, U72.P5
- new net SDA_OUT24: J147.3, J148.3, R198.1, U75.P5
- new net SDA_OUT3: J21.3, J22.3, R30.1, U12.P5
- new net SDA_OUT4: J27.3, J28.3, R38.1, U15.P5
- new net SDA_OUT5: J33.3, J34.3, R46.1, U18.P5
- new net SDA_OUT6: J39.3, J40.3, R54.1, U21.P5
- new net SDA_OUT7: J45.3, J46.3, R62.1, U24.P5
- new net SDA_OUT8: J51.3, J52.3, R70.1, U27.P5
- new net SDA_OUT9: J57.3, J58.3, R78.1, U30.P5
- net 3.3V: now also R8.2, U3.P2
- net 3.3V1: now also R16.2, U4.8, U5.5, U6.P2; no longer U3.8, U4.5
- net 3.3V10: now also R88.2, U31.8, U32.5, U33.P2; no longer U21.8, U22.5
- net 3.3V11: now also R96.2, U34.8, U35.5, U36.P2; no longer U23.8, U24.5
- net 3.3V12: now also R104.2, U37.8, U38.5, U39.P2; no longer U25.8, U26.5
- net 3.3V13: now also R112.2, U40.8, U41.5, U42.P2; no longer U27.8, U28.5
- net 3.3V14: now also R120.2, U43.8, U44.5, U45.P2; no longer U29.8, U30.5
- net 3.3V15: now also R128.2, U46.8, U47.5, U48.P2; no longer U31.8, U32.5
- net 3.3V16: now also R136.2, U49.8, U50.5, U51.P2; no longer U33.8, U34.5
- net 3.3V17: now also R144.2, U52.8, U53.5, U54.P2; no longer U35.8, U36.5
- net 3.3V18: now also R152.2, U55.8, U56.5, U57.P2; no longer U37.8, U38.5
- net 3.3V19: now also R160.2, U58.8, U59.5, U60.P2; no longer U39.8, U40.5
- net 3.3V2: now also R24.2, U7.8, U8.5, U9.P2; no longer U5.8, U6.5
- net 3.3V20: now also R168.2, U61.8, U62.5, U63.P2; no longer U41.8, U42.5
- net 3.3V21: now also R176.2, U64.8, U65.5, U66.P2; no longer U43.8, U44.5
- net 3.3V22: now also R184.2, U67.8, U68.5, U69.P2; no longer U45.8, U46.5
- net 3.3V23: now also R192.2, U70.8, U71.5, U72.P2; no longer U47.8, U48.5
- net 3.3V24: now also R200.2, U73.8, U74.5, U75.P2; no longer U49.8, U50.5
- net 3.3V3: now also R32.2, U10.8, U11.5, U12.P2; no longer U7.8, U8.5
- net 3.3V4: now also R40.2, U13.8, U14.5, U15.P2; no longer U10.5, U9.8
- net 3.3V5: now also R48.2, U16.8, U17.5, U18.P2; no longer U11.8, U12.5
- net 3.3V6: now also R56.2, U19.8, U20.5, U21.P2; no longer U13.8, U14.5
- net 3.3V7: now also R64.2, U22.8, U23.5, U24.P2; no longer U15.8, U16.5
- net 3.3V8: now also R72.2, U25.8, U26.5, U27.P2; no longer U17.8, U18.5
- net 3.3V9: now also R80.2, U28.8, U29.5, U30.P2; no longer U19.8, U20.5
- net GND: now also U3.P1
- net GND1: now also U4.4, U5.3, U6.P1; no longer U3.4, U4.3
- net GND10: now also U31.4, U32.3, U33.P1; no longer U21.4, U22.3
- net GND11: now also U34.4, U35.3, U36.P1; no longer U23.4, U24.3
- net GND12: now also U37.4, U38.3, U39.P1; no longer U25.4, U26.3
- net GND13: now also U40.4, U41.3, U42.P1; no longer U27.4, U28.3
- net GND14: now also U43.4, U44.3, U45.P1; no longer U29.4, U30.3
- net GND15: now also U46.4, U47.3, U48.P1; no longer U31.4, U32.3
- net GND16: now also U49.4, U50.3, U51.P1; no longer U33.4, U34.3
- net GND17: now also U52.4, U53.3, U54.P1; no longer U35.4, U36.3
- net GND18: now also U55.4, U56.3, U57.P1; no longer U37.4, U38.3
- net GND19: now also U58.4, U59.3, U60.P1; no longer U39.4, U40.3
- net GND2: now also U7.4, U8.3, U9.P1; no longer U5.4, U6.3
- net GND20: now also U61.4, U62.3, U63.P1; no longer U41.4, U42.3
- net GND21: now also U64.4, U65.3, U66.P1; no longer U43.4, U44.3
- net GND22: now also U67.4, U68.3, U69.P1; no longer U45.4, U46.3
- net GND23: now also U70.4, U71.3, U72.P1; no longer U47.4, U48.3
- net GND24: now also U73.4, U74.3, U75.P1; no longer U49.4, U50.3
- net GND3: now also U10.4, U11.3, U12.P1; no longer U7.4, U8.3
- net GND4: now also U13.4, U14.3, U15.P1; no longer U10.3, U9.4
- net GND5: now also U16.4, U17.3, U18.P1; no longer U11.4, U12.3
- net GND6: now also U19.4, U20.3, U21.P1; no longer U13.4, U14.3
- net GND7: now also U22.4, U23.3, U24.P1; no longer U15.4, U16.3
- net GND8: now also U25.4, U26.3, U27.P1; no longer U17.4, U18.3
- net GND9: now also U28.4, U29.3, U30.P1; no longer U19.4, U20.3
- net GPIO10: now also J18.1, U7.3; no longer J23.1, U7.2
- net GPIO11: now also U7.5, U9.P8; no longer J24.1, U7.3
- net GPIO12: now also U10.1, U11.2; no longer U10.2, U9.1
- net GPIO13: now also J23.1, U10.2; no longer J29.1, U9.2
- net GPIO14: now also J24.1, U10.3; no longer J30.1, U9.3
- net GPIO15: now also U10.5, U12.P8; no longer U11.1, U12.2
- net GPIO16: now also U13.1, U14.2; no longer J35.1, U11.2
- net GPIO17: now also J29.1, U13.2; no longer J36.1, U11.3
- net GPIO18: now also J30.1, U13.3; no longer U13.1, U14.2
- net GPIO19: now also U13.5, U15.P8; no longer J41.1, U13.2
- net GPIO20: now also U16.1, U17.2; no longer J42.1, U13.3
- net GPIO21: now also J35.1; no longer U15.1
- net GPIO22: now also J36.1, U16.3; no longer J47.1, U15.2
- net GPIO23: now also U16.5, U18.P8; no longer J48.1, U15.3
- net GPIO24: now also U19.1, U20.2; no longer U17.1, U18.2
- net GPIO25: now also J41.1, U19.2; no longer J53.1, U17.2
- net GPIO26: now also J42.1, U19.3; no longer J54.1, U17.3
- net GPIO27: now also U19.5, U21.P8; no longer U19.1, U20.2
- net GPIO28: now also U22.1, U23.2; no longer J59.1, U19.2
- net GPIO29: now also J47.1, U22.2; no longer J60.1, U19.3
- net GPIO3: now also U2.5, U3.P8; no longer U3.1, U4.2
- net GPIO30: now also J48.1, U22.3; no longer U21.1, U22.2
- net GPIO31: now also U22.5, U24.P8; no longer J65.1, U21.2
- net GPIO32: now also U25.1, U26.2; no longer J66.1, U21.3
- net GPIO33: now also J53.1, U25.2; no longer U23.1, U24.2
- net GPIO34: now also J54.1, U25.3; no longer J71.1, U23.2
- net GPIO35: now also U25.5, U27.P8; no longer J72.1, U23.3
- net GPIO36: now also U28.1, U29.2; no longer U25.1, U26.2
- net GPIO37: now also J59.1, U28.2; no longer J77.1, U25.2
- net GPIO38: now also J60.1, U28.3; no longer J78.1, U25.3
- net GPIO39: now also U28.5, U30.P8; no longer U27.1, U28.2
- net GPIO4: now also U4.1, U5.2; no longer J11.1, U3.2
- net GPIO40: now also U31.1, U32.2; no longer J83.1, U27.2
- net GPIO41: now also J65.1, U31.2; no longer J84.1, U27.3
- net GPIO42: now also J66.1, U31.3; no longer U29.1, U30.2
- net GPIO43: now also U31.5, U33.P8; no longer J89.1, U29.2
- net GPIO44: now also U34.1, U35.2; no longer J90.1, U29.3
- net GPIO45: now also J71.1, U34.2; no longer U31.1, U32.2
- net GPIO46: now also J72.1, U34.3; no longer J95.1, U31.2
- net GPIO47: now also U34.5, U36.P8; no longer J96.1, U31.3
- net GPIO48: now also U37.1, U38.2; no longer U33.1, U34.2
- net GPIO49: now also J77.1, U37.2; no longer J101.1, U33.2
- net GPIO5: now also J11.1, U4.2; no longer J12.1, U3.3
- net GPIO50: now also J78.1, U37.3; no longer J102.1, U33.3
- net GPIO51: now also U37.5, U39.P8; no longer U35.1, U36.2
- net GPIO52: now also U40.1, U41.2; no longer J107.1, U35.2
- net GPIO53: now also J83.1, U40.2; no longer J108.1, U35.3
- net GPIO54: now also J84.1, U40.3; no longer U37.1, U38.2
- net GPIO55: now also U40.5, U42.P8; no longer J113.1, U37.2
- net GPIO56: now also U43.1, U44.2; no longer J114.1, U37.3
- net GPIO57: now also J89.1, U43.2; no longer U39.1, U40.2
- net GPIO58: now also J90.1, U43.3; no longer J119.1, U39.2
- net GPIO59: now also U43.5, U45.P8; no longer J120.1, U39.3
- net GPIO6: now also J12.1, U4.3; no longer U5.1, U6.2
- net GPIO60: now also U46.1, U47.2; no longer U41.1, U42.2
- net GPIO61: now also J95.1, U46.2; no longer J125.1, U41.2
- net GPIO62: now also J96.1, U46.3; no longer J126.1, U41.3
- net GPIO63: now also U46.5, U48.P8; no longer U43.1, U44.2
- net GPIO64: now also U49.1, U50.2; no longer J131.1, U43.2
- net GPIO65: now also J101.1, U49.2; no longer J132.1, U43.3
- net GPIO66: now also J102.1, U49.3; no longer U45.1, U46.2
- net GPIO67: now also U49.5, U51.P8; no longer J137.1, U45.2
- net GPIO68: now also U52.1, U53.2; no longer J138.1, U45.3
- net GPIO69: now also J107.1, U52.2; no longer U47.1, U48.2
- net GPIO7: now also U4.5, U6.P8; no longer J17.1, U5.2
- net GPIO70: now also J108.1, U52.3; no longer J143.1, U47.2
- net GPIO71: now also U52.5, U54.P8; no longer J144.1, U47.3
- net GPIO72: now also U55.1, U56.2; no longer U49.1, U50.2
- net GPIO73: now also J113.1, U55.2; no longer J149.1, U49.2
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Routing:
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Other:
- board text added: "X02"
- board text removed: "X01"
